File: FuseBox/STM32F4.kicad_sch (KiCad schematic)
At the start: 27 parts, among them J2 702462004, J3 702462004, J4 702462004, J5 702462004, U3 STM32F407VGTx, X1 STDCSU18M

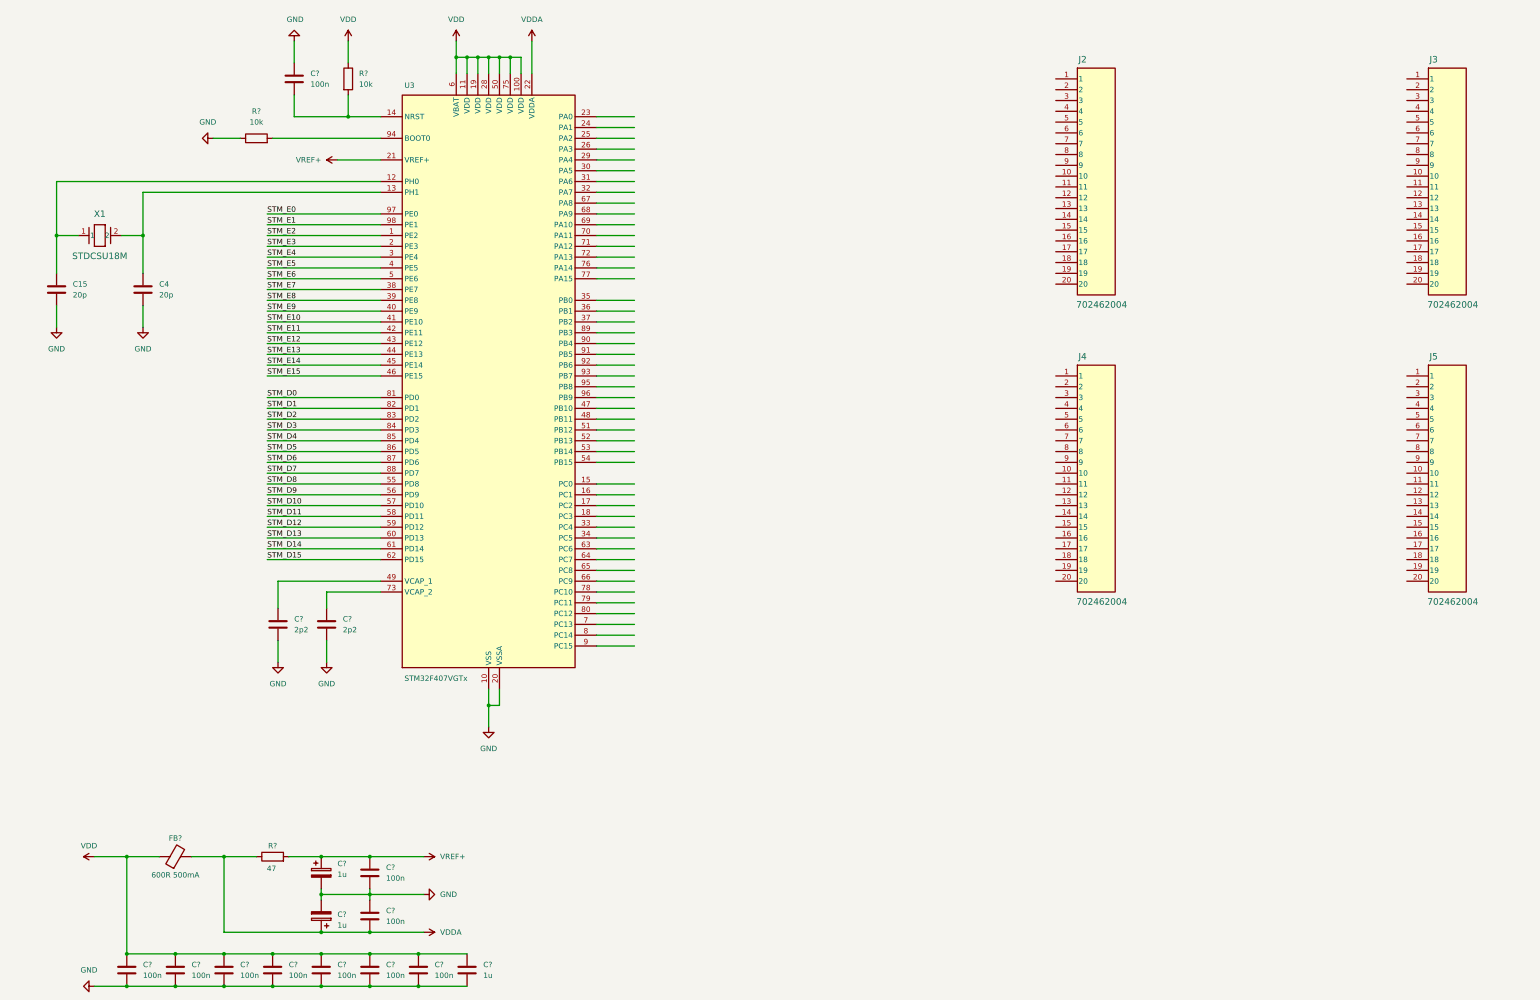
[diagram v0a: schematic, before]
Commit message: changes
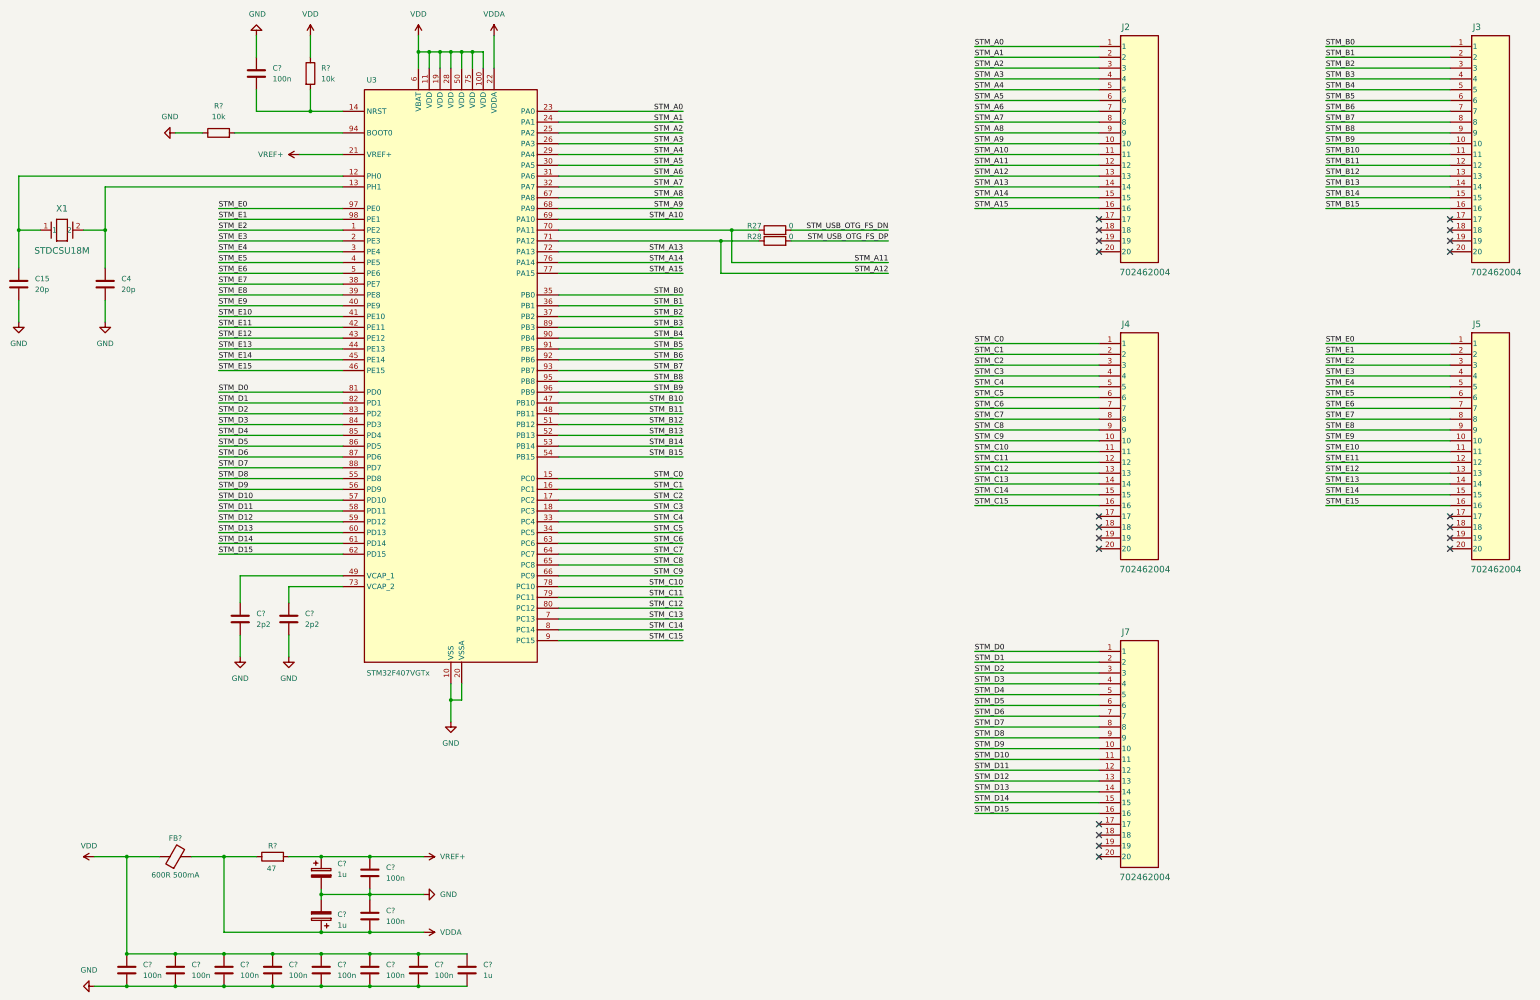
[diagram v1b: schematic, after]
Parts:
- added J7: 702462004, Custom:702462004, symbol Custom:702462004
- added R27, R28: 0, symbol Device:R
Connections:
- net STM_D0: now also J7.1
- net STM_D1: now also J7.2
- net STM_D10: now also J7.11
- net STM_D11: now also J7.12
- net STM_D12: now also J7.13
- net STM_D13: now also J7.14
- net STM_D14: now also J7.15
- net STM_D15: now also J7.16
- net STM_D2: now also J7.3
- net STM_D3: now also J7.4
- net STM_D4: now also J7.5
- net STM_D5: now also J7.6
- net STM_D6: now also J7.7
- net STM_D7: now also J7.8
- net STM_D8: now also J7.9
- net STM_D9: now also J7.10
- net STM_E0: now also J5.1
- net STM_E1: now also J5.2
- net STM_E10: now also J5.11
- net STM_E11: now also J5.12
- net STM_E12: now also J5.13
- net STM_E13: now also J5.14
- net STM_E14: now also J5.15
- net STM_E15: now also J5.16
- net STM_E2: now also J5.3
- net STM_E3: now also J5.4
- net STM_E4: now also J5.5
- net STM_E5: now also J5.6
- net STM_E6: now also J5.7
- net STM_E7: now also J5.8
- net STM_E8: now also J5.9
- net STM_E9: now also J5.10
- net STM_A0: now reaches J2.1
- net STM_A0: now also U3.23 (PA0)
- net STM_A9: now reaches J2.10
- net STM_A9: now also U3.68 (PA9)
- net STM_A10: now reaches J2.11
- net STM_A10: now also U3.69 (PA10)
- net STM_A11: now reaches J2.12
- net STM_A11: now also U3.70 (PA11), R27.1
- net STM_A12: now reaches J2.13
- net STM_A12: now also U3.71 (PA12), R28.1
- net STM_A13: now reaches J2.14
- net STM_A13: now also U3.72 (PA13)
- net STM_A14: now reaches J2.15
- net STM_A14: now also U3.76 (PA14)
- net STM_A15: now reaches J2.16
- net STM_A15: now also U3.77 (PA15)
- net STM_A1: now reaches J2.2
- net STM_A1: now also U3.24 (PA1)
- net STM_A2: now reaches J2.3
- net STM_A2: now also U3.25 (PA2)
- net STM_A3: now reaches J2.4
- net STM_A3: now also U3.26 (PA3)
- net STM_A4: now reaches J2.5
- net STM_A4: now also U3.29 (PA4)
- net STM_A5: now reaches J2.6
- net STM_A5: now also U3.30 (PA5)
- net STM_A6: now reaches J2.7
- net STM_A6: now also U3.31 (PA6)
- net STM_A7: now reaches J2.8
- net STM_A7: now also U3.32 (PA7)
- net STM_A8: now reaches J2.9
- net STM_A8: now also U3.67 (PA8)
- net STM_C0: now reaches U3.15 (PC0)
- net STM_C0: now also J4.1
- net STM_C1: now reaches U3.16 (PC1)
- net STM_C1: now also J4.2
- net STM_C2: now reaches U3.17 (PC2)
- net STM_C2: now also J4.3
- net STM_C3: now reaches U3.18 (PC3)
- net STM_C3: now also J4.4
- net STM_C4: now reaches U3.33 (PC4)
- net STM_C4: now also J4.5
- net STM_C5: now reaches U3.34 (PC5)
- net STM_C5: now also J4.6
- net STM_B0: now reaches U3.35 (PB0)
- net STM_B0: now also J3.1
- net STM_B1: now reaches U3.36 (PB1)
- net STM_B1: now also J3.2
- net STM_B2: now reaches U3.37 (PB2)
- net STM_B2: now also J3.3
- net STM_B10: now reaches U3.47 (PB10)
- net STM_B10: now also J3.11
- net STM_B11: now reaches U3.48 (PB11)
- net STM_B11: now also J3.12
- net STM_B12: now reaches U3.51 (PB12)
- net STM_B12: now also J3.13
- net STM_B13: now reaches U3.52 (PB13)
- net STM_B13: now also J3.14
- net STM_B14: now reaches U3.53 (PB14)
- net STM_B14: now also J3.15
- net STM_B15: now reaches U3.54 (PB15)
- net STM_B15: now also J3.16
- net STM_C6: now reaches U3.63 (PC6)
- net STM_C6: now also J4.7
- net STM_C7: now reaches U3.64 (PC7)
- net STM_C7: now also J4.8
- net STM_C8: now reaches U3.65 (PC8)
- net STM_C8: now also J4.9
- net STM_C9: now reaches U3.66 (PC9)
- net STM_C9: now also J4.10
- net STM_C13: now reaches U3.7 (PC13)
- net STM_C13: now also J4.14
- net STM_C10: now reaches U3.78 (PC10)
- net STM_C10: now also J4.11
- net STM_C11: now reaches U3.79 (PC11)
- net STM_C11: now also J4.12
- net STM_C14: now reaches U3.8 (PC14)
- net STM_C14: now also J4.15
- net STM_C12: now reaches U3.80 (PC12)
- net STM_C12: now also J4.13
- net STM_B3: now reaches U3.89 (PB3)
- net STM_B3: now also J3.4
- net STM_C15: now reaches U3.9 (PC15)
- net STM_C15: now also J4.16
- net STM_B4: now reaches U3.90 (PB4)
- net STM_B4: now also J3.5
- net STM_B5: now reaches U3.91 (PB5)
- net STM_B5: now also J3.6
- net STM_B6: now reaches U3.92 (PB6)
- net STM_B6: now also J3.7
- net STM_B7: now reaches U3.93 (PB7)
- net STM_B7: now also J3.8
- net STM_B8: now reaches U3.95 (PB8)
- net STM_B8: now also J3.9
- net STM_B9: now reaches U3.96 (PB9)
- net STM_B9: now also J3.10
- new net STM_USB_OTG_FS_DN: R27.2
- new net STM_USB_OTG_FS_DP: R28.2
- no-connect marks 0 -> 20
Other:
- moved on the sheet: C15, C4, C?, J2, J3, J4, J5, R?, U3, X1

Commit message: finished schematic
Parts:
- C15, C4, C? (x15): footprint (none) -> Capacitor_SMD:C_0603_1608Metric_Pad1.08x0.95mm_HandSolder
- FB?: footprint (none) -> Inductor_SMD:L_0603_1608Metric_Pad1.05x0.95mm_HandSolder
- R27, R28, R? (x3): footprint (none) -> Resistor_SMD:R_0603_1608Metric_Pad0.98x0.95mm_HandSolder
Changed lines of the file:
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@@
 			)
 		)
-		(property "Footprint" ""
+		(property "Footprint" "Inductor_SMD:L_0603_1608Metric_Pad1.05x0.95mm_HandSolder"
 			(at 64.77 231.648 90)
 			(effects
@@
 			)
 		)
-		(property "Footprint" ""
+		(property "Footprint" "Resistor_SMD:R_0603_1608Metric_Pad0.98x0.95mm_HandSolder"
 			(at 87.63 231.648 90)
 			(effects
@@
 			)
 		)
-		(property "Footprint" ""
+		(property "Footprint" "Capacitor_SMD:C_0603_1608Metric_Pad1.08x0.95mm_HandSolder"
 			(at 54.3052 260.35 0)
 			(effects
@@
 			)
 		)
-		(property "Footprint" ""
+		(property "Footprint" "Capacitor_SMD:C_0603_1608Metric_Pad1.08x0.95mm_HandSolder"
 			(at 134.3152 260.35 0)
 			(effects
@@
 			)
 		)
-		(property "Footprint" ""
+		(property "Footprint" "Capacitor_SMD:C_0603_1608Metric_Pad1.08x0.95mm_HandSolder"
 			(at 100.0252 237.49 0)
 			(effects
@@
 			)
 		)
-		(property "Footprint" ""
+		(property "Footprint" "Capacitor_SMD:C_0603_1608Metric_Pad1.08x0.95mm_HandSolder"
 			(at 26.9748 91.44 0)
 			(effects
@@
 			)
 		)
-		(property "Footprint" ""
+		(property "Footprint" "Capacitor_SMD:C_0603_1608Metric_Pad1.08x0.95mm_HandSolder"
 			(at 82.8548 41.91 0)
 			(effects
@@
 			)
 		)
-		(property "Footprint" ""
+		(property "Footprint" "Capacitor_SMD:C_0603_1608Metric_Pad1.08x0.95mm_HandSolder"
 			(at 65.7352 260.35 0)
 			(effects
@@
 			)
 		)
-		(property "Footprint" ""
+		(property "Footprint" "Capacitor_SMD:C_0603_1608Metric_Pad1.08x0.95mm_HandSolder"
 			(at 111.4552 237.49 0)
 			(effects
@@
 			)
 		)
-		(property "Footprint" ""
+		(property "Footprint" "Capacitor_SMD:C_0603_1608Metric_Pad1.08x0.95mm_HandSolder"
 			(at 111.4552 247.65 0)
 			(effects
@@
 			)
 		)
-		(property "Footprint" ""
+		(property "Footprint" "Capacitor_SMD:C_0603_1608Metric_Pad1.08x0.95mm_HandSolder"
 			(at 111.4552 260.35 0)
 			(effects
@@
 			)
 		)
-		(property "Footprint" ""
+		(property "Footprint" "Capacitor_SMD:C_0603_1608Metric_Pad1.08x0.95mm_HandSolder"
 			(at 92.4052 177.8 0)
 			(effects
@@
 			)
 		)
-		(property "Footprint" ""
+		(property "Footprint" "Capacitor_SMD:C_0603_1608Metric_Pad1.08x0.95mm_HandSolder"
 			(at 47.2948 91.44 0)
 			(effects
@@
 			)
 		)
-		(property "Footprint" ""
+		(property "Footprint" "Resistor_SMD:R_0603_1608Metric_Pad0.98x0.95mm_HandSolder"
 			(at 74.93 61.468 90)
 			(effects
@@
 			)
 		)
-		(property "Footprint" ""
+		(property "Footprint" "Capacitor_SMD:C_0603_1608Metric_Pad1.08x0.95mm_HandSolder"
 			(at 98.0948 240.03 0)
 			(effects
@@
 			)
 		)
-		(property "Footprint" ""
+		(property "Footprint" "Capacitor_SMD:C_0603_1608Metric_Pad1.08x0.95mm_HandSolder"
 			(at 77.1652 260.35 0)
 			(effects
@@
 			)
 		)
-		(property "Footprint" ""
+		(property "Footprint" "Resistor_SMD:R_0603_1608Metric_Pad0.98x0.95mm_HandSolder"
 			(at 205.74 84.328 90)
 			(effects
@@
 			)
 		)
-		(property "Footprint" ""
+		(property "Footprint" "Capacitor_SMD:C_0603_1608Metric_Pad1.08x0.95mm_HandSolder"
 			(at 100.0252 260.35 0)
 			(effects
@@
 			)
 		)
-		(property "Footprint" ""
+		(property "Footprint" "Capacitor_SMD:C_0603_1608Metric_Pad1.08x0.95mm_HandSolder"
 			(at 80.9752 177.8 0)
 			(effects
@@
 			)
 		)
-		(property "Footprint" ""
+		(property "Footprint" "Resistor_SMD:R_0603_1608Metric_Pad0.98x0.95mm_HandSolder"
 			(at 205.74 86.868 90)
 			(effects
@@
 			)
 		)
-		(property "Footprint" ""
+		(property "Footprint" "Capacitor_SMD:C_0603_1608Metric_Pad1.08x0.95mm_HandSolder"
 			(at 88.5952 260.35 0)
 			(effects
@@
 			)
 		)
-		(property "Footprint" ""
+		(property "Footprint" "Resistor_SMD:R_0603_1608Metric_Pad0.98x0.95mm_HandSolder"
 			(at 94.742 45.72 90)
 			(effects
@@
 			)
 		)
-		(property "Footprint" ""
+		(property "Footprint" "Capacitor_SMD:C_0603_1608Metric_Pad1.08x0.95mm_HandSolder"
 			(at 122.8852 260.35 0)
 			(effects
